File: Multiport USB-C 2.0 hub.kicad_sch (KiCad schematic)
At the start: 0 parts

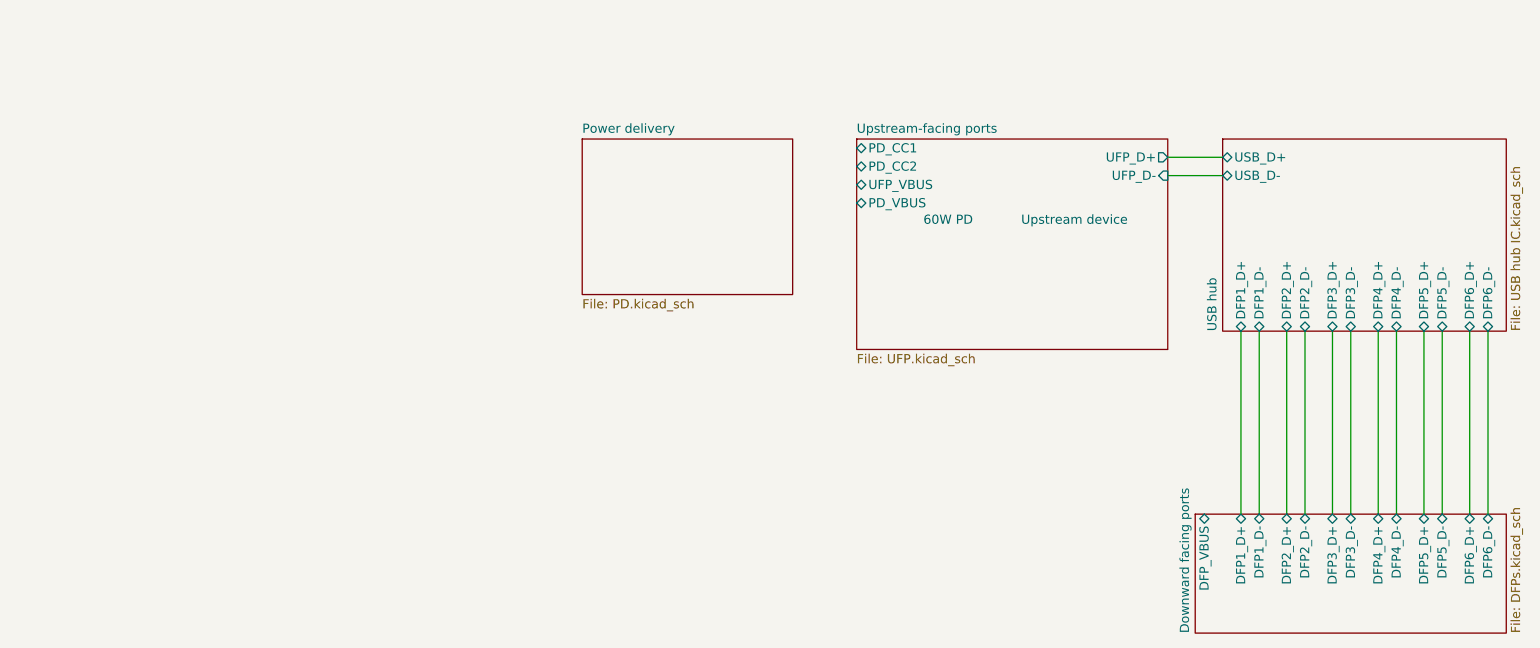
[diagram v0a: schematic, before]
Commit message: good first pass
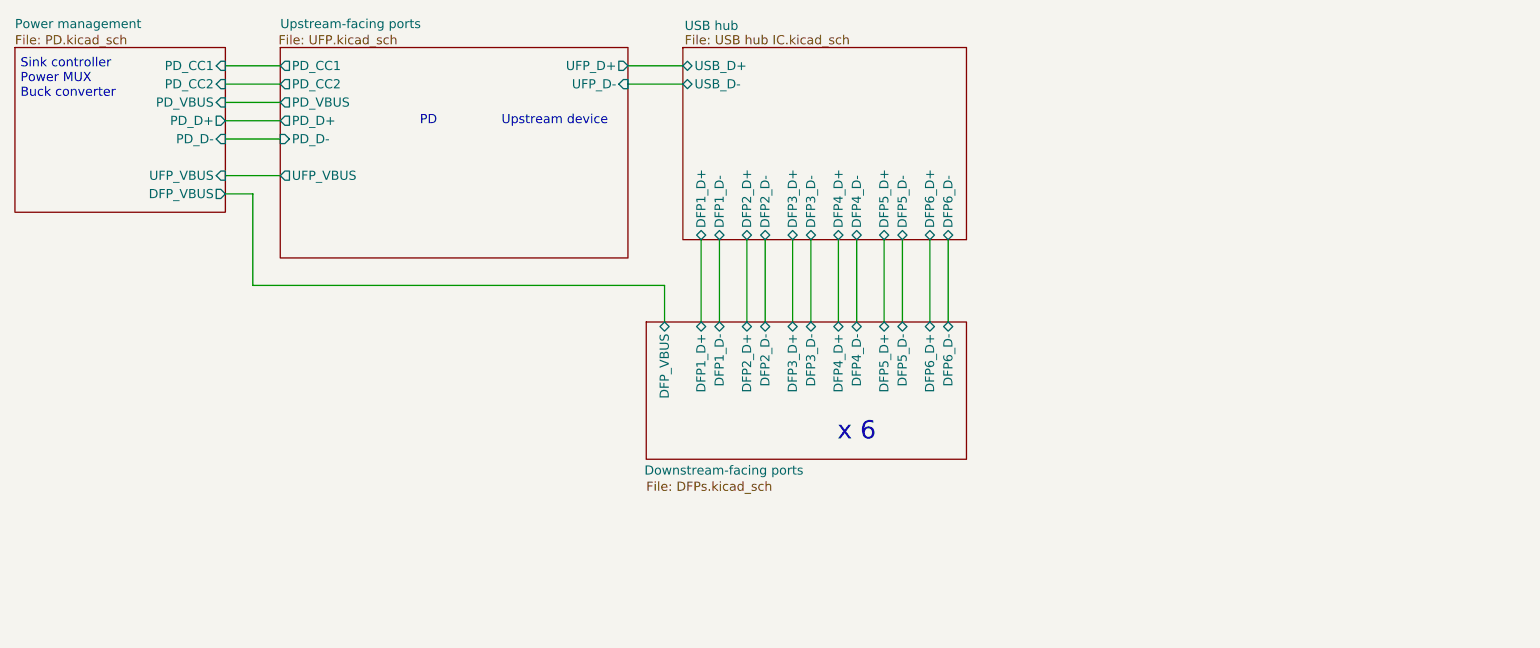
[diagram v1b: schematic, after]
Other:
- sheet Downward facing ports renamed Downstream-facing ports
- sheet Power delivery renamed Power management
- sheet Power management ports: added DFP_VBUS, PD_CC1, PD_CC2, PD_D+, PD_D-, PD_VBUS, UFP_VBUS; removed none
- sheet Upstream-facing ports ports: added PD_D+, PD_D-; removed none
- note added: "PD"
- note added: "Sink controller Power MUX Buck converter"
- note added: "x 6"
- note removed: "60W PD"
- company: (none) -> https://pips.engineering
- title: (none) -> Multiport USB-C 2.0 hub
